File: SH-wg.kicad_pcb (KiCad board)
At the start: 4 copper layers, 54.6 x 79.2 mm, 73 parts, among them J101 Aux PCB Conn Male, J102 Aux PCB Conn Female, J201 Conn_01x05, J301 JTAG, J302 Digital IO, J303 Analog IO, J401 Power, J501 Conn_01x04, J701 Conn_02x03_Odd_Even, Q801 2N7002, U201 SN65HVD231, U301 ESP32-WROOM-32E, U601 XL1509-3.3, U801 AH1902

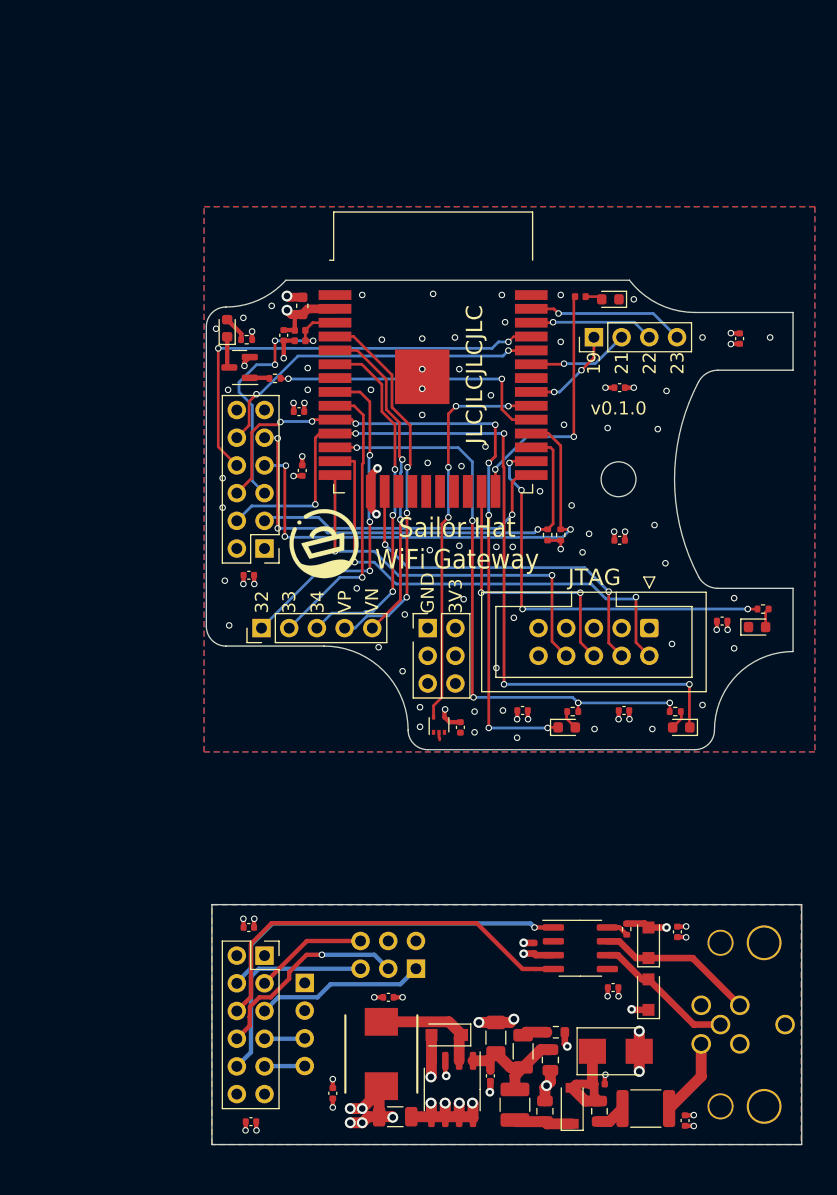
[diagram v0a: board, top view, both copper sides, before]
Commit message: Prepare final 0.1.0 proto
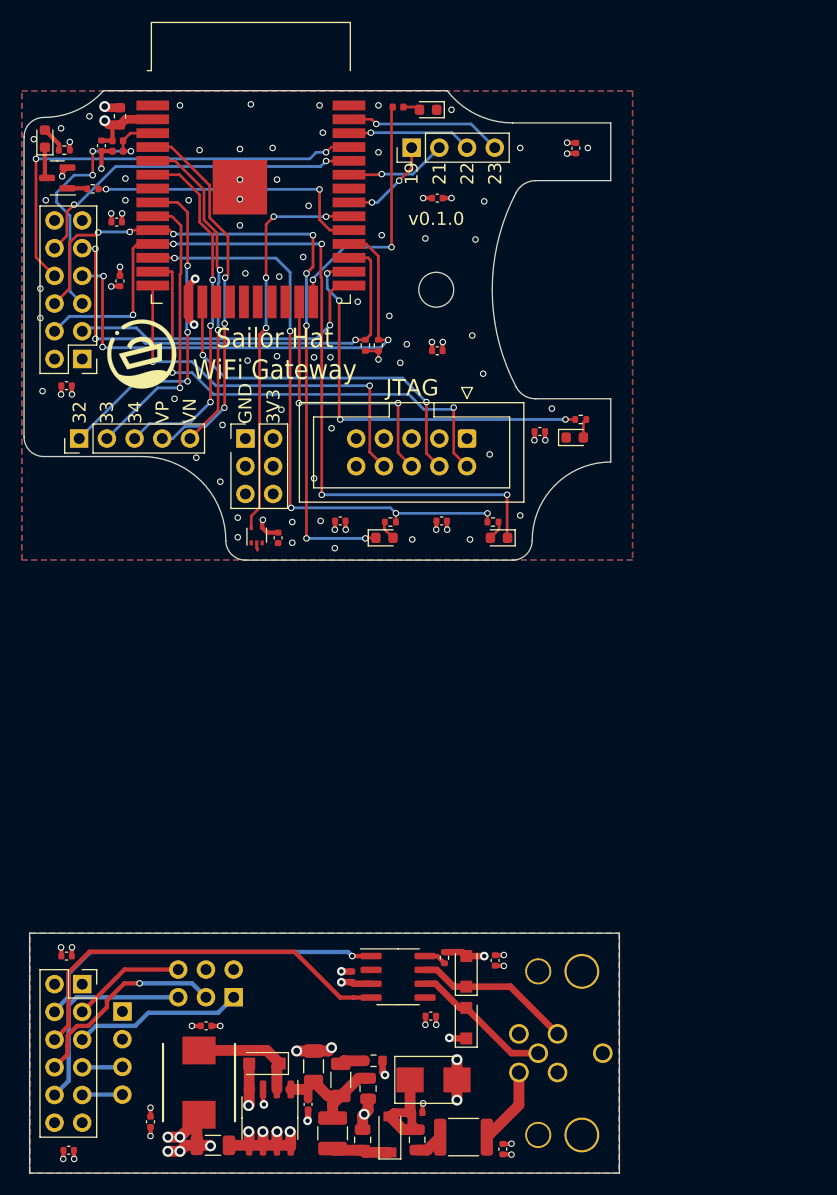
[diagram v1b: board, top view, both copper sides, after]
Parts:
- added REF**: Tab, kikit:Tab, F.Cu at (80.8, 83.8)
- added REF**: Tab, kikit:Tab, F.Cu at (42.8, 127.5)
- added REF**: Tab, kikit:Tab, F.Cu at (97.2, 127.6)
- added REF**: Tab, kikit:Tab, F.Cu at (96.5, 44.8)
- added REF**: Tab, kikit:Tab, F.Cu at (70.0, 138.8)
- added REF**: Tab, kikit:Tab, F.Cu at (77.3, 39.1)
- added REF**: Tab, kikit:Tab, F.Cu at (42.2, 57.6)
- added REF**: Tab, kikit:Tab, F.Cu at (70.0, 116.3)
- added REF**: Tab, kikit:Tab, F.Cu at (96.5, 70.5)
- D603: value SS24FL -> DSS34
- L601: value NLCV32T-100K-PFR -> CBC3225T100KR
- U201: value SN65HVD231 -> SN65HVD232DR
- moved C405 24.1 mm to (71.5, 78.8)
- moved C406 24.1 mm to (80.8, 78.8)
- moved R801 24.1 mm to (93.5, 69.5)
- moved U801 24.1 mm to (63.8, 80.1)
- moved C302 24.1 mm to (51.3, 41.7)
- moved C407 24.1 mm to (51.3, 56.8)
- moved D802 24.1 mm to (79.5, 41.1)
- moved G401 24.1 mm to (53.3, 63.5)
- moved H404 24.1 mm to (80.3, 57.6)
- moved J302 24.1 mm to (78.0, 44.6)
- moved Q801 24.1 mm to (45.5, 47.4)
- moved R802 24.1 mm to (76.8, 40.9)
- moved R805 24.1 mm to (48.8, 48.4)
- moved U301 24.1 mm to (63.3, 49.0)
- moved C401 24.1 mm to (51.0, 51.4)
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- renumbered H401 to H404
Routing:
- net GND: vias 78 -> 76
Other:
- board size 54.6 x 79.2 mm -> 54.6 x 99.2 mm
- board text removed: "JLCJLCJLCJLC"
